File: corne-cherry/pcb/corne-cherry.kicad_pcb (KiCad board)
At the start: 2 copper layers, 152.8 x 91.4 mm, 101 parts, among them J1 MJ-4PP-9, J2 OLED, J3 LED, P1 i2c-pin, P2 i2c-pin, SW1 SW_PUSH, SW10 SW_PUSH, SW11 SW_PUSH, SW12 SW_PUSH, SW13 SW_PUSH, SW14 SW_PUSH, SW15 SW_PUSH, SW16 SW_PUSH, SW17 SW_PUSH, SW18 SW_PUSH, SW19 SW_PUSH, SW2 SW_PUSH, SW20 SW_PUSH, SW21 SW_PUSH, SW22 SW_PUSH, SW3 SW_PUSH, SW4 SW_PUSH, SW5 SW_PUSH, SW6 SW_PUSH, SW7 SW_PUSH, SW8 SW_PUSH, SW9 SW_PUSH, U1 ProMicro

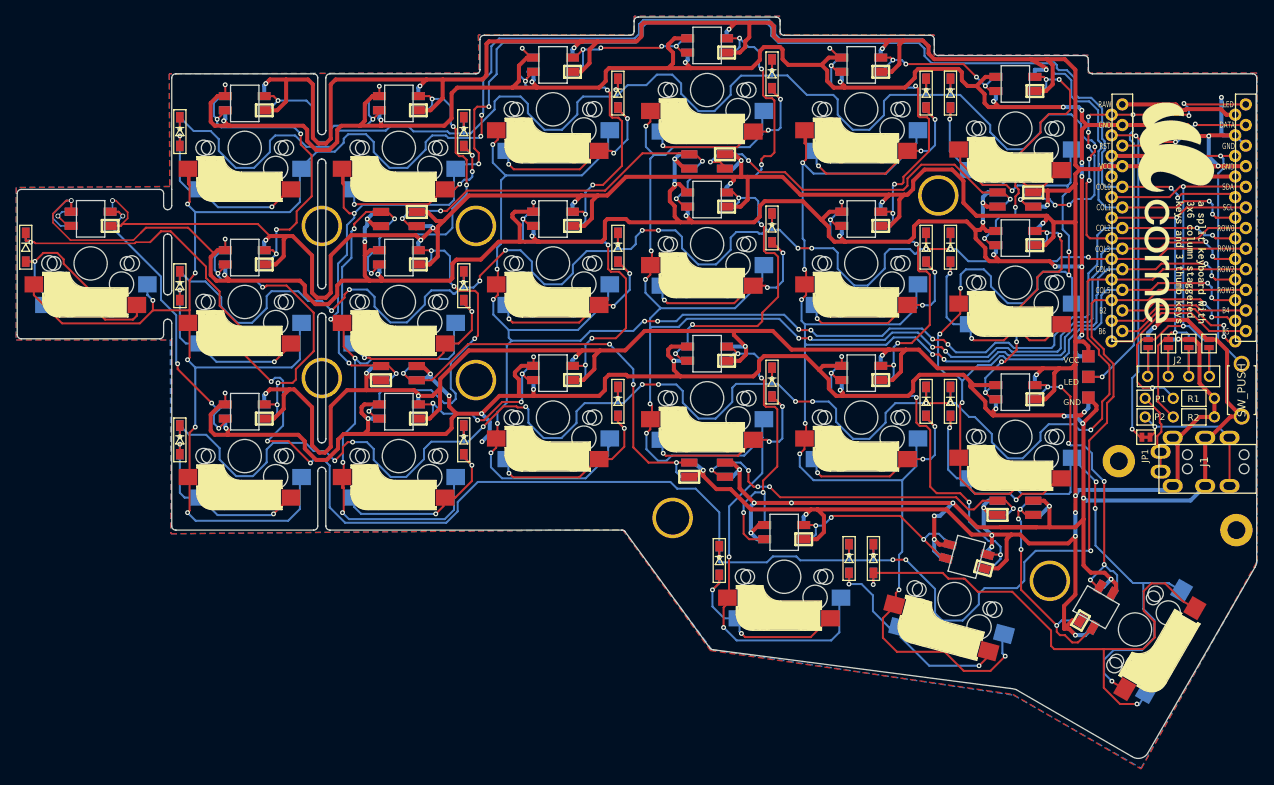
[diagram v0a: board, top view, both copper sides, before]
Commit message: Clean
Clean up
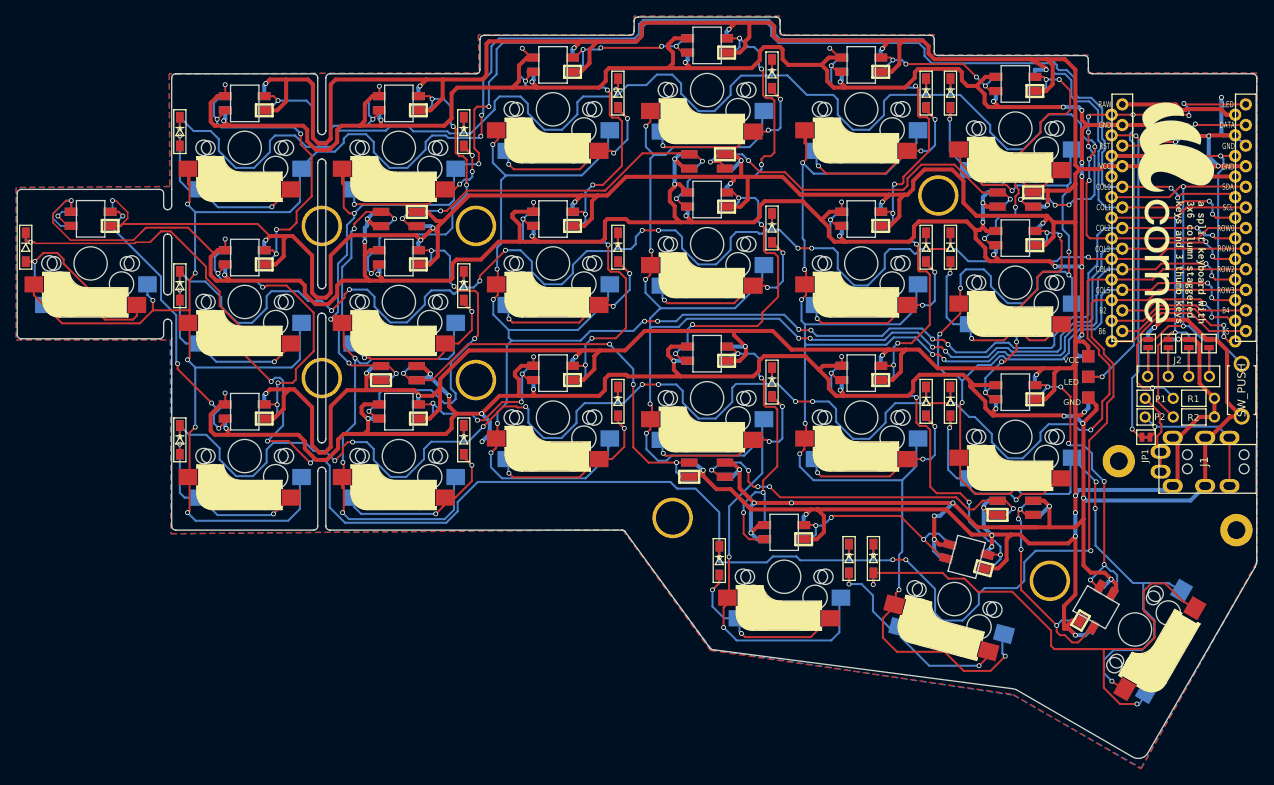
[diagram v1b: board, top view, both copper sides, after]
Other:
- net class Default removed
- net class Power removed
